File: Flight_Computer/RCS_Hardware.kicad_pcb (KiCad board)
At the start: 2 copper layers, 50.8 x 50 mm, 57 parts, among them J1 SWD, J2 TYPE-C-31-M-12, J3 JST BATT, J4 3V3, J5 GND, J6 Solenoids, J7 Ext Sesnor, J8 Conn_01x05_Male, U1 STM32F401CCU6, U2 AMS1117-3.3, U3 BMP280, U4 BNO055, U5 W25Q32JVSS, U6 AMS1117-3.3, U7 LT1690N8, Y1 16MHz, Y2 32.768Mhz

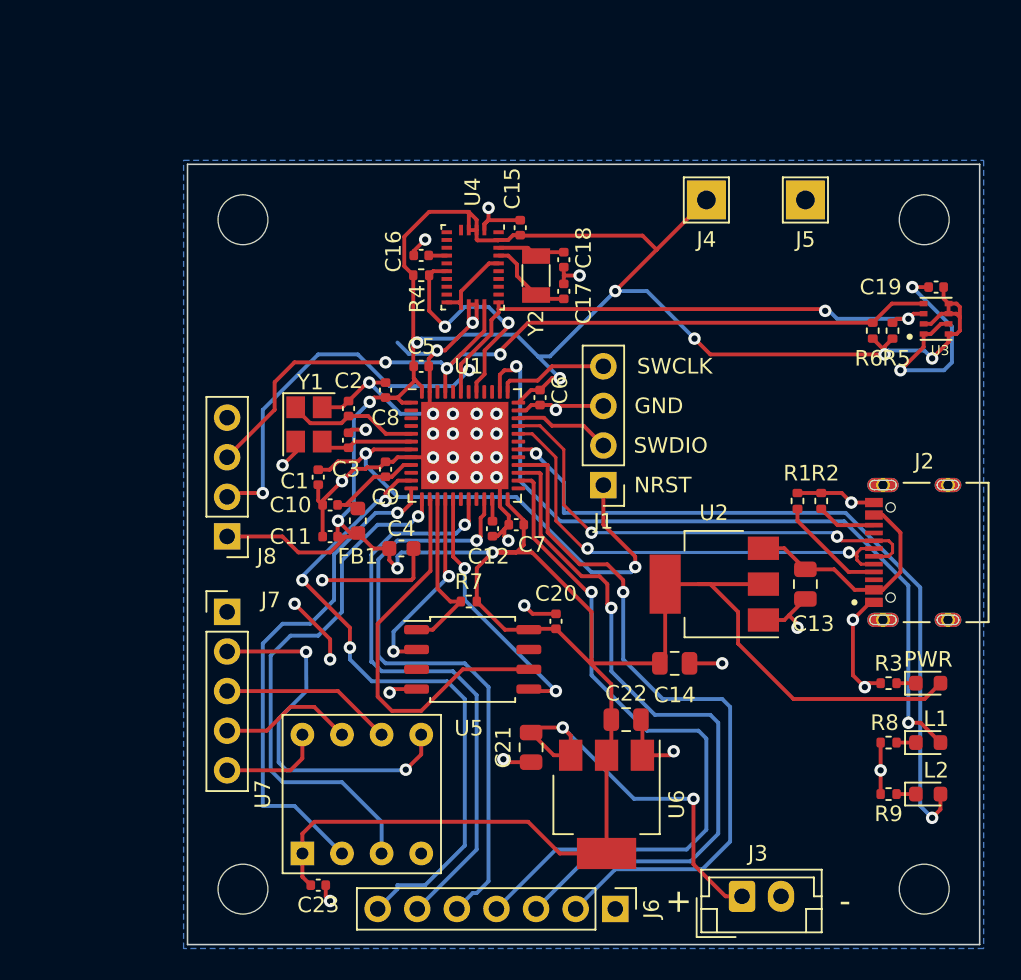
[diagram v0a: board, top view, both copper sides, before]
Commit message: started new routing
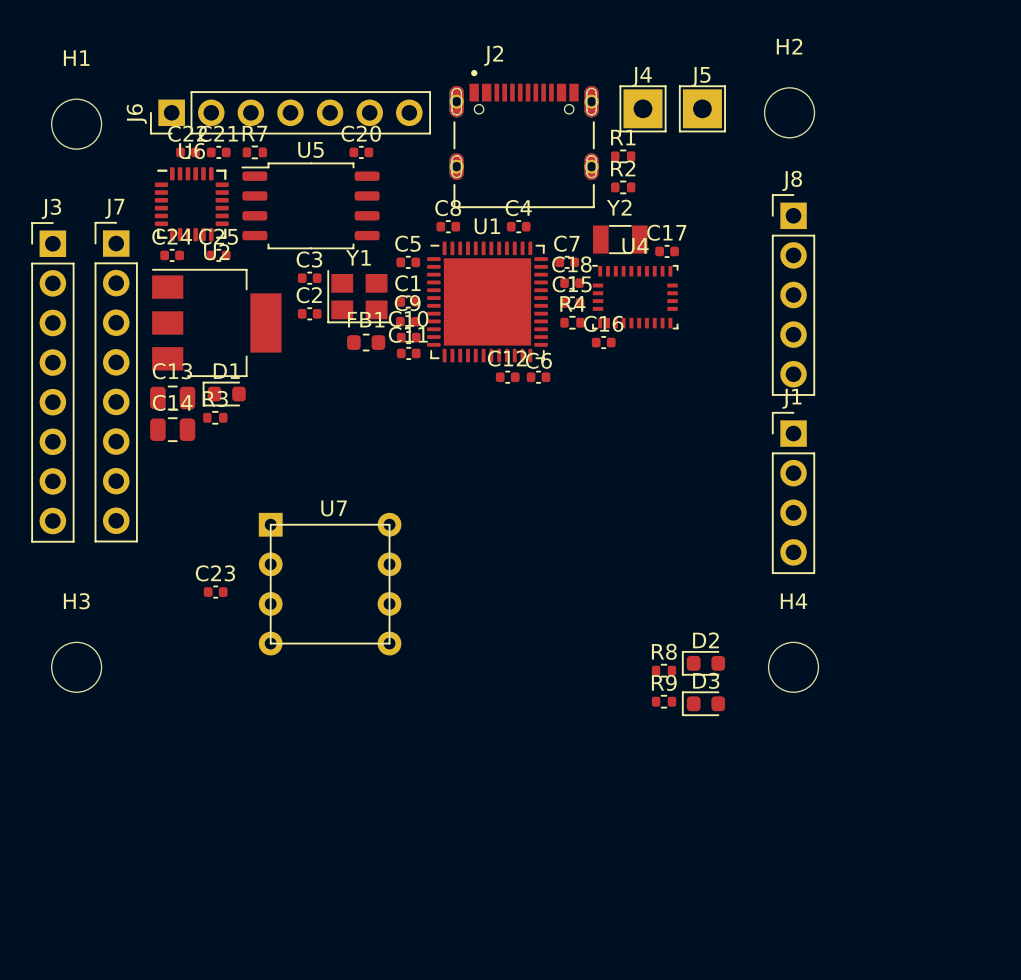
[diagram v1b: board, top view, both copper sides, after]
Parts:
- removed C19: 100nF, Capacitor_SMD:C_0402_1005Metric
- removed R5, R6: 10k, Resistor_SMD:R_0402_1005Metric
- removed U3: BMP280, BMP280:XDCR_BMP280
- added C24: 0.1uF, Capacitor_SMD:C_0402_1005Metric, F.Cu at (110.3, 80.3)
- added C25: 10nF, Capacitor_SMD:C_0402_1005Metric, F.Cu at (113.3, 80.3)
- C21: value 22uF -> 0.1uF; footprint Capacitor_SMD:C_0805_2012Metric -> Capacitor_SMD:C_0402_1005Metric
- C22: value 22uF -> 2.2nF; footprint Capacitor_SMD:C_0805_2012Metric -> Capacitor_SMD:C_0402_1005Metric
- C4: footprint Capacitor_SMD:C_0603_1608Metric -> Capacitor_SMD:C_0402_1005Metric
- J3: value JST BATT -> SPI; footprint Connector_JST:JST_EH_B2B-EH-A_1x02_P2.50mm_Vertical -> Connector_PinHeader_2.54mm:PinHeader_1x08_P2.54mm_Vertical
- J4: value 3V3 -> 5V
- J7: value Ext Sesnor -> SPI; footprint Connector_PinHeader_2.54mm:PinHeader_1x04_P2.54mm_Vertical -> Connector_PinHeader_2.54mm:PinHeader_1x08_P2.54mm_Vertical
- U6: value AMS1117-3.3 -> MPU-6050; footprint Package_TO_SOT_SMD:SOT-223-3_TabPin2 -> Sensor_Motion:InvenSense_QFN-24_4x4mm_P0.5mm
- U7: value LT1690N8 -> LTC1690N8
- moved H1 73.2 mm to (104.1, 71.8)
- moved J3 60.9 mm to (102.6, 79.5)
- moved J6 58.4 mm to (110.2, 71.1), turned to 90 degrees
- moved D1 48.7 mm to (113.8, 89.2)
- moved U6 46.8 mm to (111.5, 77.0), turned to 0 degrees
- moved R3 46.4 mm to (113.0, 90.7), turned to 0 degrees
- moved C22 46.0 mm to (111.3, 73.7)
- moved H4 45.5 mm to (150.1, 106.7)
- moved J8 44.3 mm to (150.1, 77.7)
- moved C21 43.1 mm to (113.3, 73.7), turned to 0 degrees
- moved C13 42.3 mm to (110.3, 89.4), turned to 0 degrees
- moved J2 36.8 mm to (132.8, 74.6), turned to 0 degrees
- moved U2 36.0 mm to (113.1, 84.6), turned to 0 degrees
- moved C14 35.5 mm to (110.3, 91.4)
- moved C20 32.6 mm to (122.4, 73.7), turned to 0 degrees
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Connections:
- C21 pad 1: /BATT_IN -> Net-(U6-REGOUT)
- C22 pad 1: +3.3V -> Net-(U6-CPOUT)
- C23 pad 1: +3.3V -> VBUS
- J3 pad 1: /BATT_IN -> /CS1
- J3 pad 2: GND -> /MOSI2
- J4 pad 1: +3.3V -> VBUS
- J7 pad 1: +3.3V -> /CS2
- J7 pad 2: /SDA -> /MOSI2
- J7 pad 3: /SCL -> /MISO2
- J7 pad 4: GND -> /SCK
- U6 pad 1: GND -> /CLKIN
- U6 pad 2: +3.3V -> unconnected-(U6-NC-Pad2)
- U6 pad 3: /BATT_IN -> unconnected-(U6-NC-Pad3)
- U7 pad 1: +3.3V -> VBUS
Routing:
- net +3.3V: track 234.1 -> 0.00 mm, vias 10 -> 0
- net GND: track 126.7 -> 0.00 mm, vias 43 -> 0
- net /SDA: track 59.7 -> 0.00 mm, vias 4 -> 0
- net /SCL: track 56.9 -> 0.00 mm, vias 3 -> 0
- net /LED_G: track 49.0 -> 0.00 mm, vias 2 -> 0
- net /LED_B: track 47.5 -> 0.00 mm, vias 2 -> 0
- net /S6: track 45.8 -> 0.00 mm, vias 1 -> 0
- net /S5: track 45.7 -> 0.00 mm, vias 1 -> 0
- net /S4: track 45.5 -> 0.00 mm, vias 1 -> 0
- net /S1: track 41.6 -> 0.00 mm, vias 3 -> 0
- net /S3: track 39.0 -> 0.00 mm, vias 1 -> 0
- net /S2: track 38.3 -> 0.00 mm, vias 1 -> 0
- net /TX: track 34.2 -> 0.00 mm, vias 1 -> 0
- net /NRST: track 33.7 -> 0.00 mm, vias 2 -> 0
- net /RX: track 32.7 -> 0.00 mm, vias 1 -> 0
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- removed copper zone on B.Cu, net GND
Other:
- board size 50.8 x 50 mm -> 9.2 x 5.7 mm
- board text removed: "+"
- board text removed: "-"
- board text removed: "GND"
- board text removed: "L1"
- board text removed: "L2"
- board text removed: "NRST"
- board text removed: "SARP RCS Flight Computer V1.0"
- board text removed: "SWCLK"
- board text removed: "SWDIO"
